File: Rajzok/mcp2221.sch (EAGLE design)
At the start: 17 parts, among them Q1 TP0602N2, Q2 TP0602N2, Q3 SUP75N06-08, Q4 SUP75N06-08

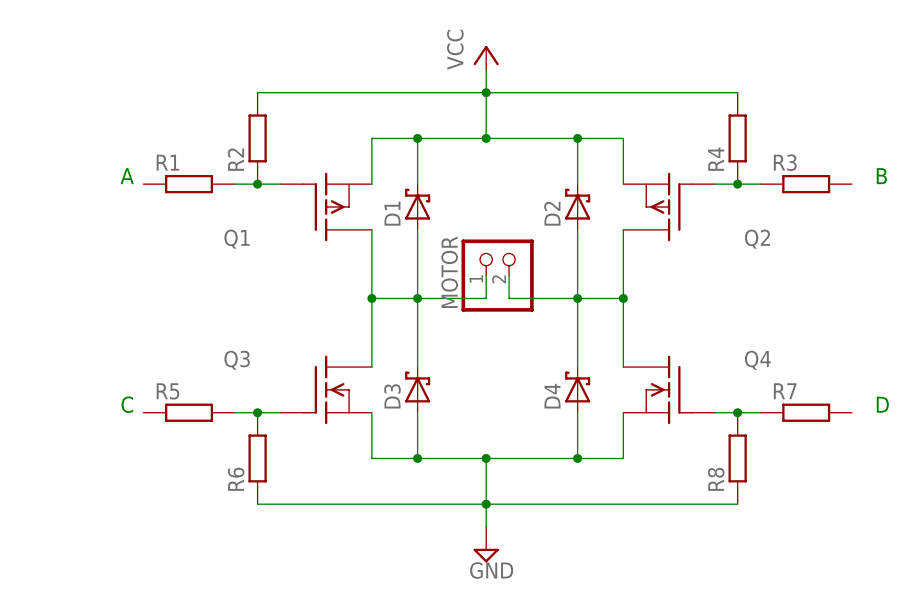
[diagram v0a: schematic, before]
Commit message: Rajzok 2017
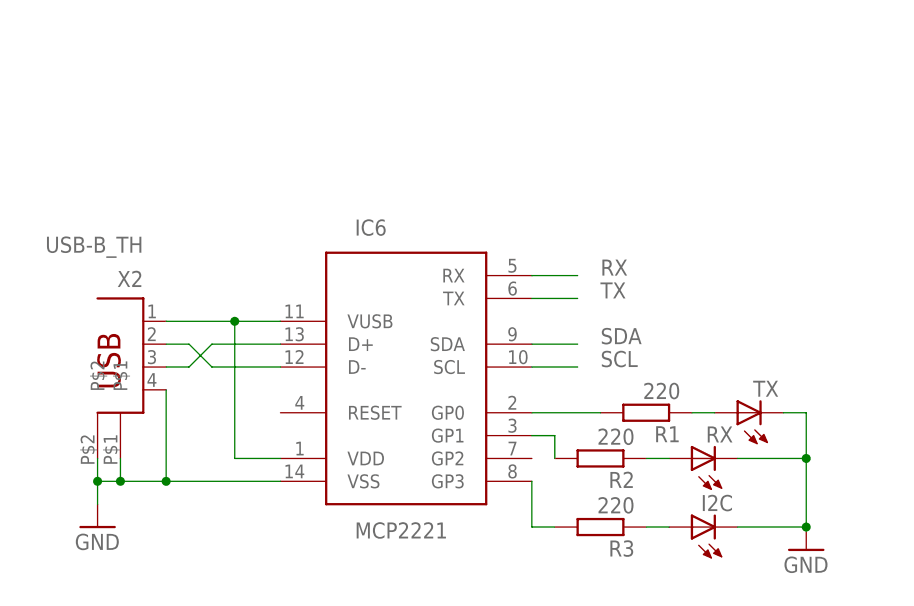
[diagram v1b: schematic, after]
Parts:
- removed D1, D2, D3, D4: 1N6267A, diode:1N6267A
- removed MOTOR: (no value), pinhead:PINHD-1X2
- removed Q1, Q2: TP0602N2, transistor-fet:TP0602N2
- removed Q3, Q4: SUP75N06-08, transistor-fet:SUP75N06-08
- removed R4, R5, R6, R7, R8: (no value), rcl:R-EU_0204/7
- added I2C, RX, TX: (no value), led:LED5MM
- added IC6: MCP2221, Webmaster442:MCP2221
- added X2: USB-B_TH, SmartPrj:PN61729
- R1, R2, R3: value (none) -> 220; device rcl:R-EU_0204/7 -> rcl:R-EU_0207/10
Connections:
- removed net N$4: Q3.G, R5.2, R6.2
- removed net N$9: D1.A, D3.C, MOTOR.1, Q1.D, Q3.D
- removed net VCC: D1.C, D2.C, Q1.S, Q2.S, R2.2, R4.2
- new net LED_RX: IC6.GP0, R1.2
- new net LED_TX: IC6.GP1, R2.2
- new net N$10: IC6.D-, X2.2
- new net N$27: IC6.D+, X2.3
- new net RX: IC6.RX
- new net SCL: IC6.SCL
- new net SDA: IC6.SDA
- new net TX: IC6.TX
- new net VCORE: IC6.VDD, IC6.VUSB, X2.1
- net GND: now also I2C.C, IC6.VSS, RX.C, TX.C, X2.4, X2.P$1, X2.P$2; no longer D3.A, D4.A, Q3.S, Q4.S, R6.1, R8.1
- net N$1: now also R1.1, TX.A; no longer Q1.G, R1.2, R2.1
- net N$2: now also R2.1, RX.A; no longer D2.A, D4.C, MOTOR.2, Q2.D, Q4.D
- net N$3: now also I2C.A; no longer Q2.G, R4.1
- net N$5: now also IC6.GP3, R3.2; no longer Q4.G, R7.1, R8.2
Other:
- note removed: "A"
- note removed: "B"
- note removed: "C"
- note removed: "D"
- moved on the sheet: R1, R2, R3
